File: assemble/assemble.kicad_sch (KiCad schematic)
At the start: 118 parts, among them SW1 SW_Push, SW10 SW_Push, SW11 SW_Push, SW12 SW_Push, SW13 SW_Push, SW14 SW_Push, SW15 SW_Push, SW16 SW_Push, SW17 SW_Push, SW18 SW_Push, SW19 SW_Push, SW2 SW_Push, SW20 SW_Push, SW21 SW_Push, SW22 SW_Push, SW23 SW_Push, SW24 SW_Push, SW25 SW_Push, SW26 SW_Push, SW27 SW_Push, SW28 SW_Push, SW29 SW_Push, SW3 SW_Push, SW30 SW_Push, SW31 SW_Push, SW32 SW_Push, SW33 SW_Push, SW34 SW_Push, SW35 SW_Push, SW36 SW_Push, SW37 SW_Push, SW38 SW_Push, SW39 SW_Push, SW4 SW_Push, SW40 SW_Push, SW41 SW_Push, SW42 SW_Push, SW43 SW_SPDT, SW44 SW_SPDT, SW45 RotaryEncoder_Switch, SW46 RotaryEncoder_Switch, SW5 SW_Push, SW6 SW_Push, SW7 SW_Push, SW8 SW_Push, SW9 SW_Push, U1 XIAO-nRF52840-SMD, U2 XIAO-nRF52840-SMD

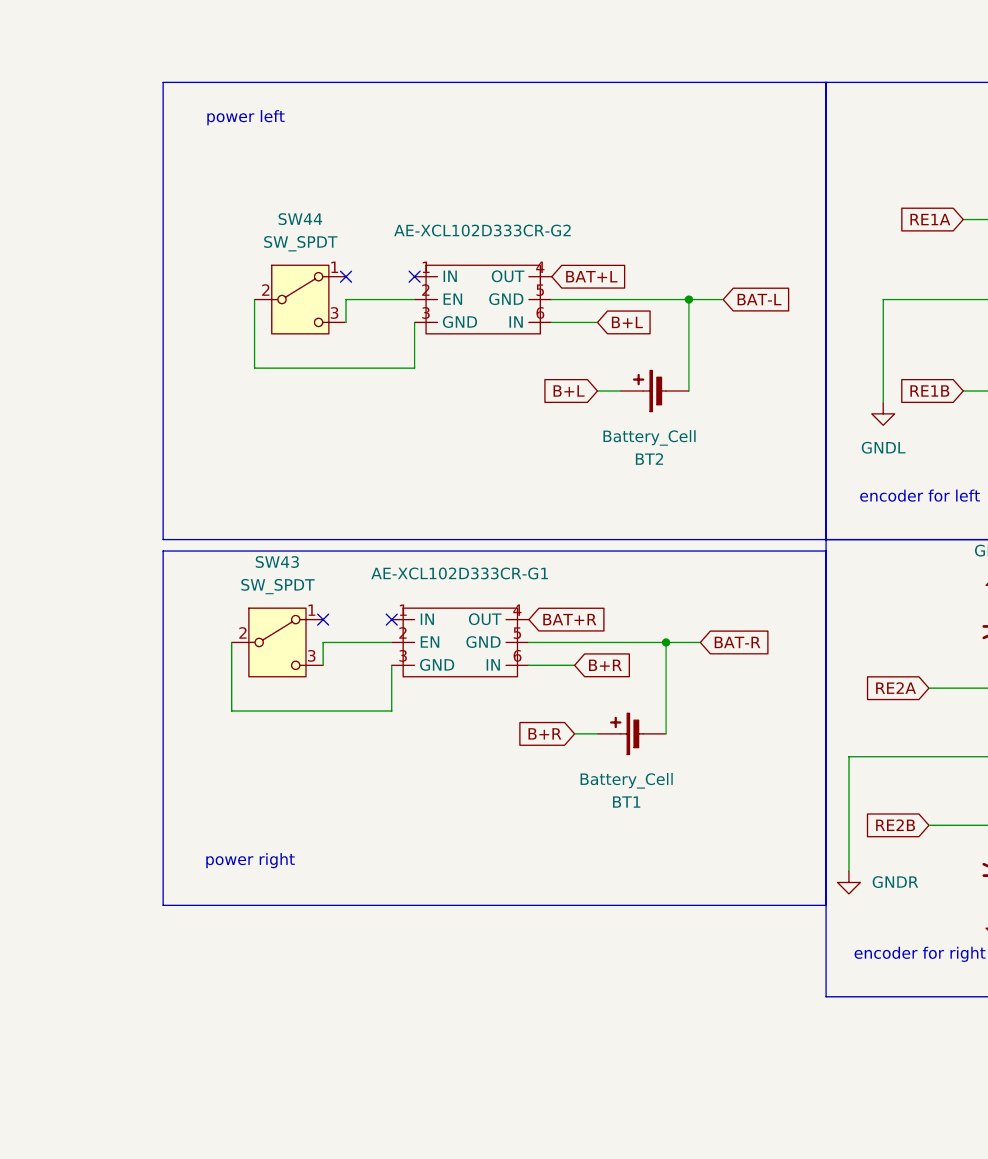
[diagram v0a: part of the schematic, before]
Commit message: wip: implement PCB
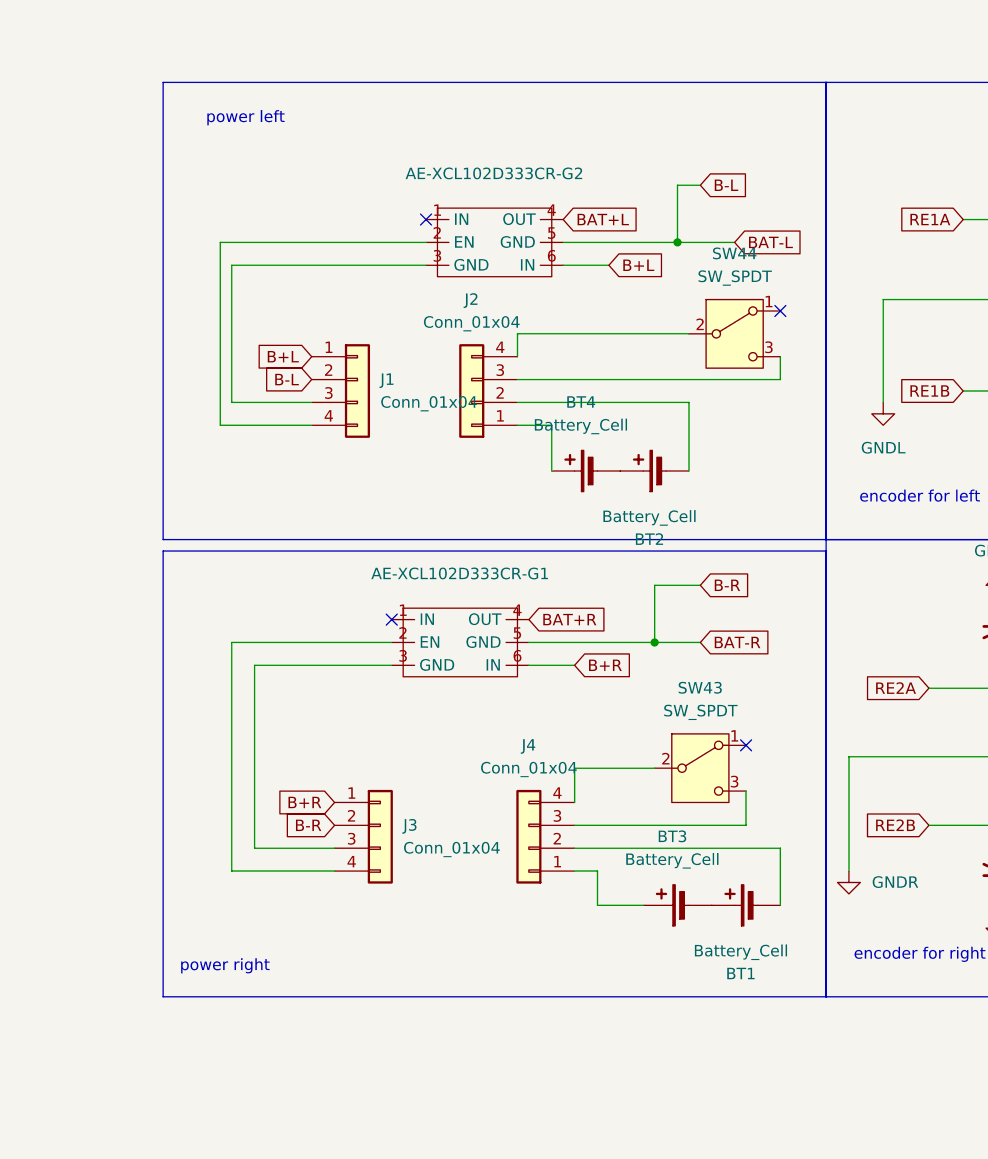
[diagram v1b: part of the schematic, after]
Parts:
- added BT3, BT4: Battery_Cell, kbd_Parts:Battery_AAA, symbol Device:Battery_Cell
- added J1, J3: Conn_01x04, Connector_JST:JST_ZH_B4B-ZR_1x04_P1.50mm_Vertical, symbol Connector_Generic:Conn_01x04
- added J2, J4: Conn_01x04, Connector_Wire:SolderWire-0.5sqmm_1x04_P4.6mm_D0.9mm_OD2.1mm, symbol Connector_Generic:Conn_01x04
- BT1, BT2: footprint Battery:BatteryHolder_Keystone_2460_1xAA -> kbd_Parts:Battery_AAA
- C1, C2, C3, C4: footprint (none) -> kbd_Parts:Capacitor_1206
- R1, R2, R3, R4: footprint (none) -> Resistor_SMD:R_0805_2012Metric_Pad1.20x1.40mm_HandSolder
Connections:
- net B+L: now also J1.1 (Pin_1); no longer BT2.1 (+)
- net B+R: now also J3.1 (Pin_1); no longer BT1.1 (+)
- net at SW43.2 (B): now also J4.4 (Pin_4); no longer AE-XCL102D333CR-G1.3 (GND)
- net at SW43.3 (C): now also J4.3 (Pin_3); no longer AE-XCL102D333CR-G1.2 (EN)
- net at SW44.3 (C): now also J2.3 (Pin_3); no longer AE-XCL102D333CR-G2.2 (EN)
- net at SW44.2 (B): now also J2.4 (Pin_4); no longer AE-XCL102D333CR-G2.3 (GND)
- net BAT-L renamed B-L
- net B-L: now also J1.2 (Pin_2); no longer BT2.2 (-)
- net BAT-R renamed B-R
- net B-R: now also J3.2 (Pin_2); no longer BT1.2 (-)
- new net: BT3.1 (+), J4.1 (Pin_1)
- new net: BT1.2 (-), J4.2 (Pin_2)
- new net: BT1.1 (+), BT3.2 (-)
- new net: BT4.1 (+), J2.1 (Pin_1)
- new net: BT2.2 (-), J2.2 (Pin_2)
- new net: BT2.1 (+), BT4.2 (-)
- new net: AE-XCL102D333CR-G2.2 (EN), J1.4 (Pin_4)
- new net: AE-XCL102D333CR-G2.3 (GND), J1.3 (Pin_3)
- new net: AE-XCL102D333CR-G1.3 (GND), J3.3 (Pin_3)
- new net: AE-XCL102D333CR-G1.2 (EN), J3.4 (Pin_4)
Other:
- moved on the sheet: AE-XCL102D333CR-G2, BT1, BT2, SW43, SW44
